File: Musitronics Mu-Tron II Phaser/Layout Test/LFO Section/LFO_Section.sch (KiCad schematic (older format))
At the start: 44 parts, among them J201 Conn_01x08, J202 Conn_01x08, J203 Conn_01x03, Q201 2N4401, U201 TL062, U202 TL071

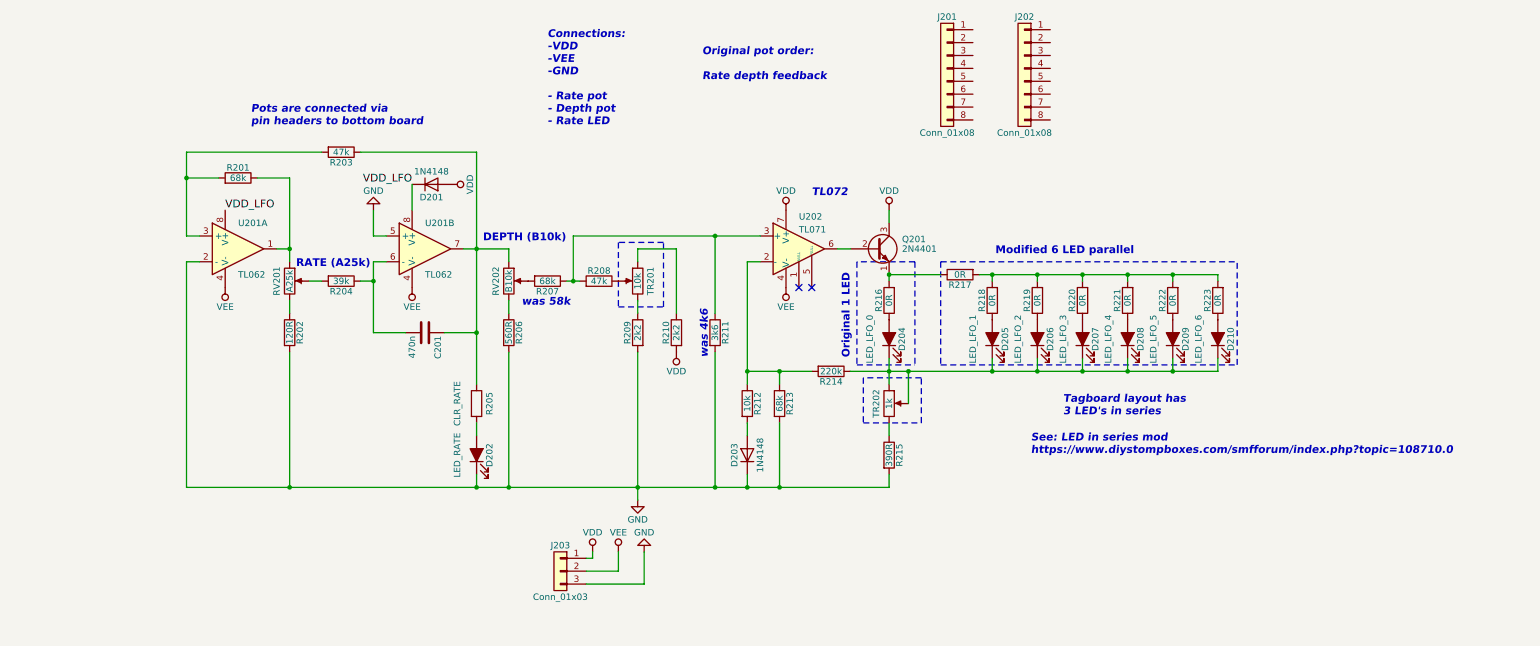
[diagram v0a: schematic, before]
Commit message: mu-tron update, bom
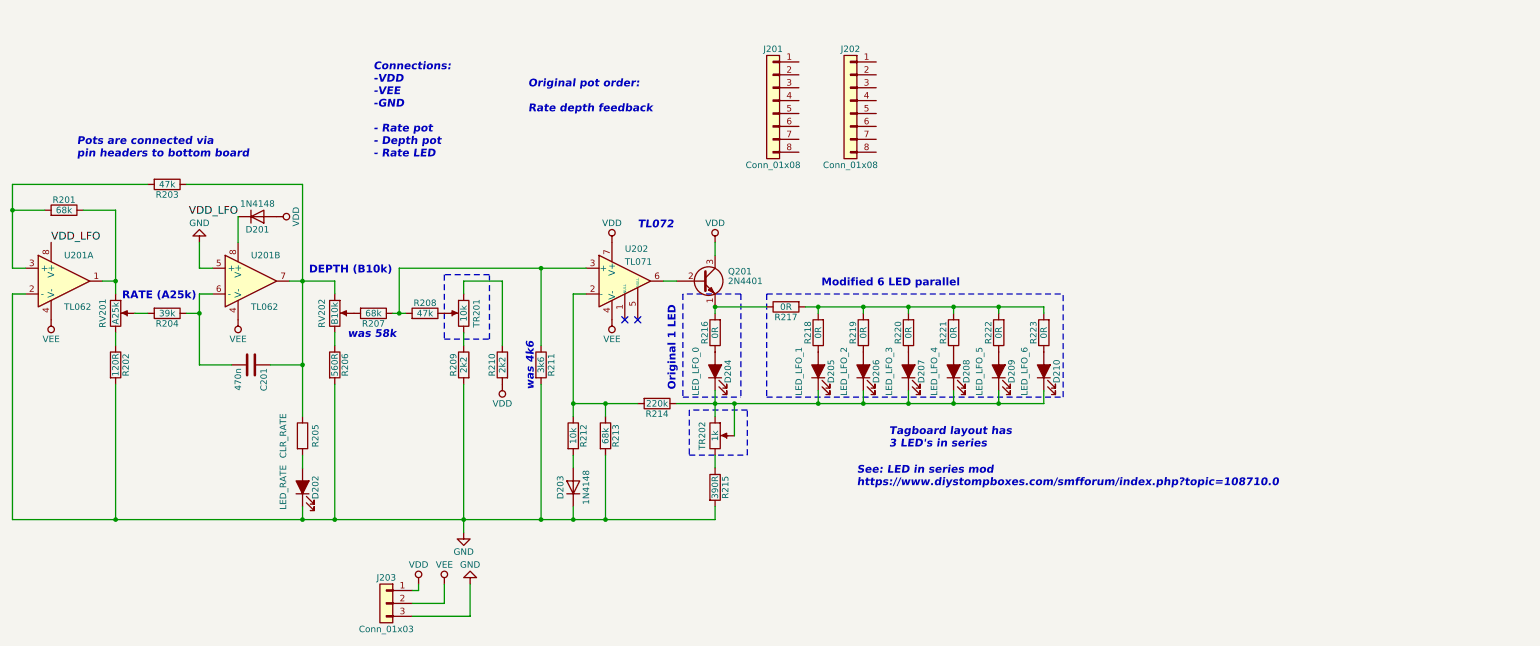
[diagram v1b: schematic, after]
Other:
- moved on the sheet: C201, D201, D202, D203, D204, D205, D206, D207, D208, D209, D210, J201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
